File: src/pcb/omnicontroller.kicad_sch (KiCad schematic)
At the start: 47 parts, among them J1 G-Switch GT-USB-7010ASV, U1 RP2040, U2 NCP1117ST33T3G, U3 W25Q128JVSIM, X1 SW_Omron_B3FS-1000P, Y1 ABM8-272-T3, Y2 SW_Omron_B3FS-1000P

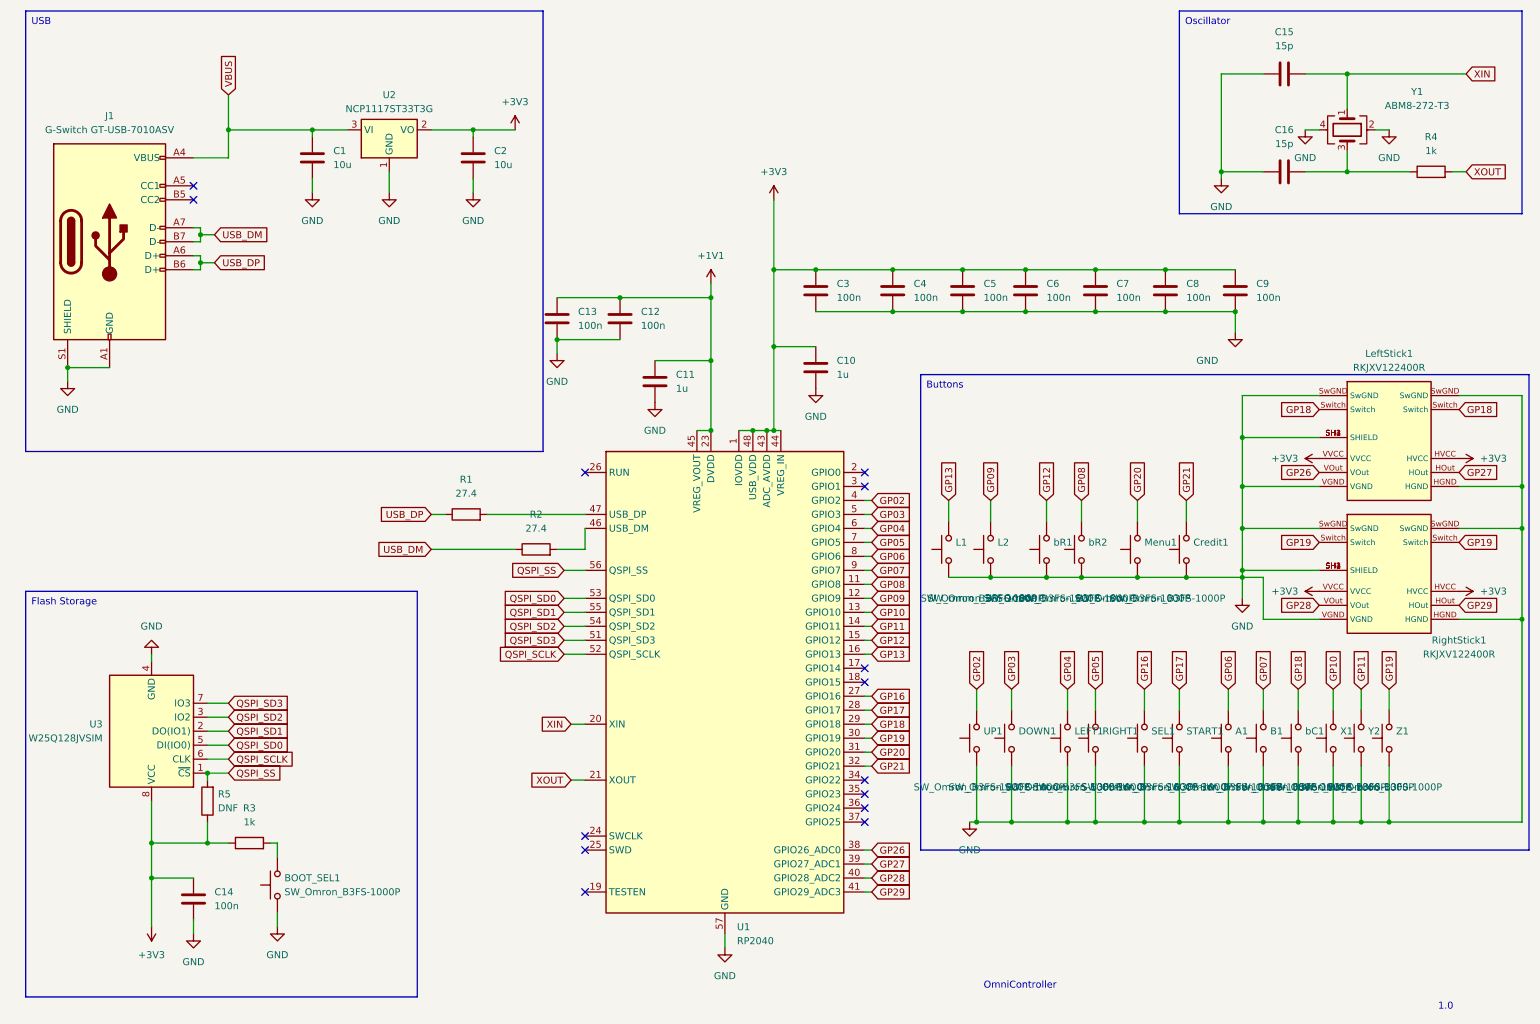
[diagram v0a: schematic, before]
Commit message: convert to kicad 9.0 file format
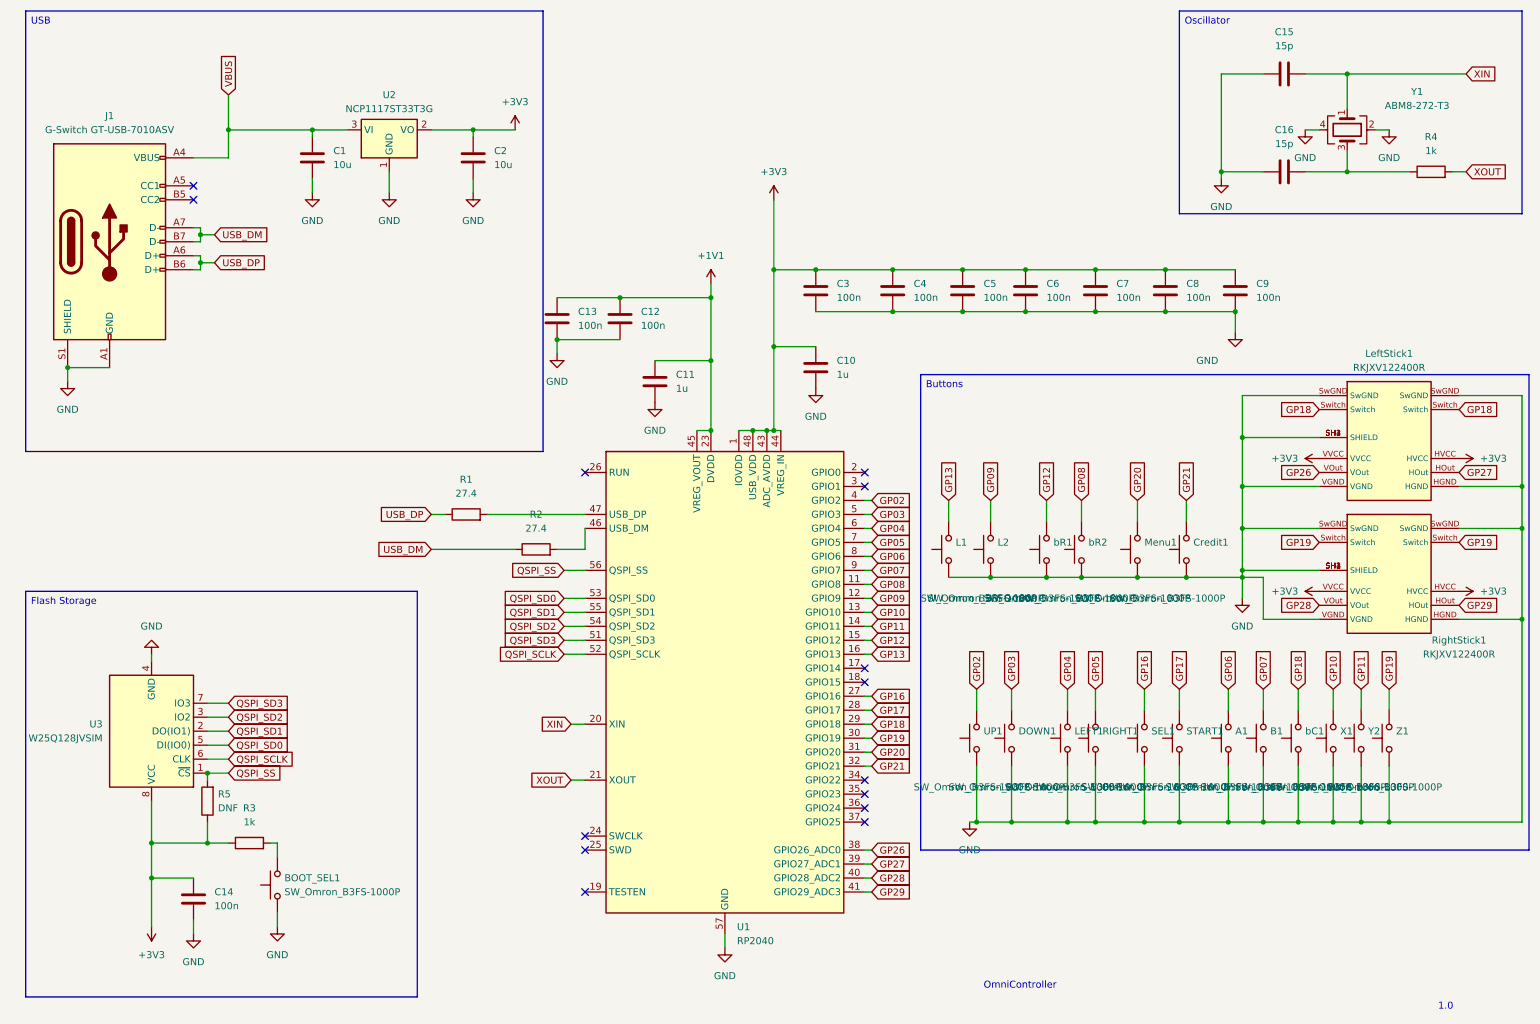
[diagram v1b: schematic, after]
